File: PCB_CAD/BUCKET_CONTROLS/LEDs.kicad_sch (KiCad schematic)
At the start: 104 parts, among them J1 Pow, J10 Data, J101 Pow, J102 Data, J103 Pow, J104 Data, J105 Pow, J106 Data, J107 Pow, J108 Data, J109 Pow, J11 Pow, J110 Data, J111 Pow, J112 Data, J113 Pow, J114 Data, J115 Pow, J116 Data, J117 Pow, J118 Data, J119 Pow, J12 Data, J120 Data, J13 Pow, J14 Pow, J15 Pow, J16 Data, J17 Data, J18 Data, J19 Pow, J2 Data, J20 Data, J201 Pow, J202 Data, J203 Pow, J204 Data, J205 Pow, J206 Data, J207 Pow, J208 Data, J209 Pow, J210 Data, J211 Pow, J212 Data, J213 Pow, J214 Data, J215 Pow, J216 Data, J217 Pow, J218 Data, J219 Pow, J220 Data, J3 Pow, J301 Pow, J302 Data, J303 Pow, J304 Data, J305 Pow, J306 Data, J307 Pow, J308 Data, J309 Pow, J310 Data, J311 Pow, J312 Data, J313 Pow, J314 Data, J315 Pow, J316 Data, J317 Pow, J318 Data, J319 Pow, J320 Data, J4 Data, J5 Pow, J6 Data, J7 Pow, J8 Pow, J9 Data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

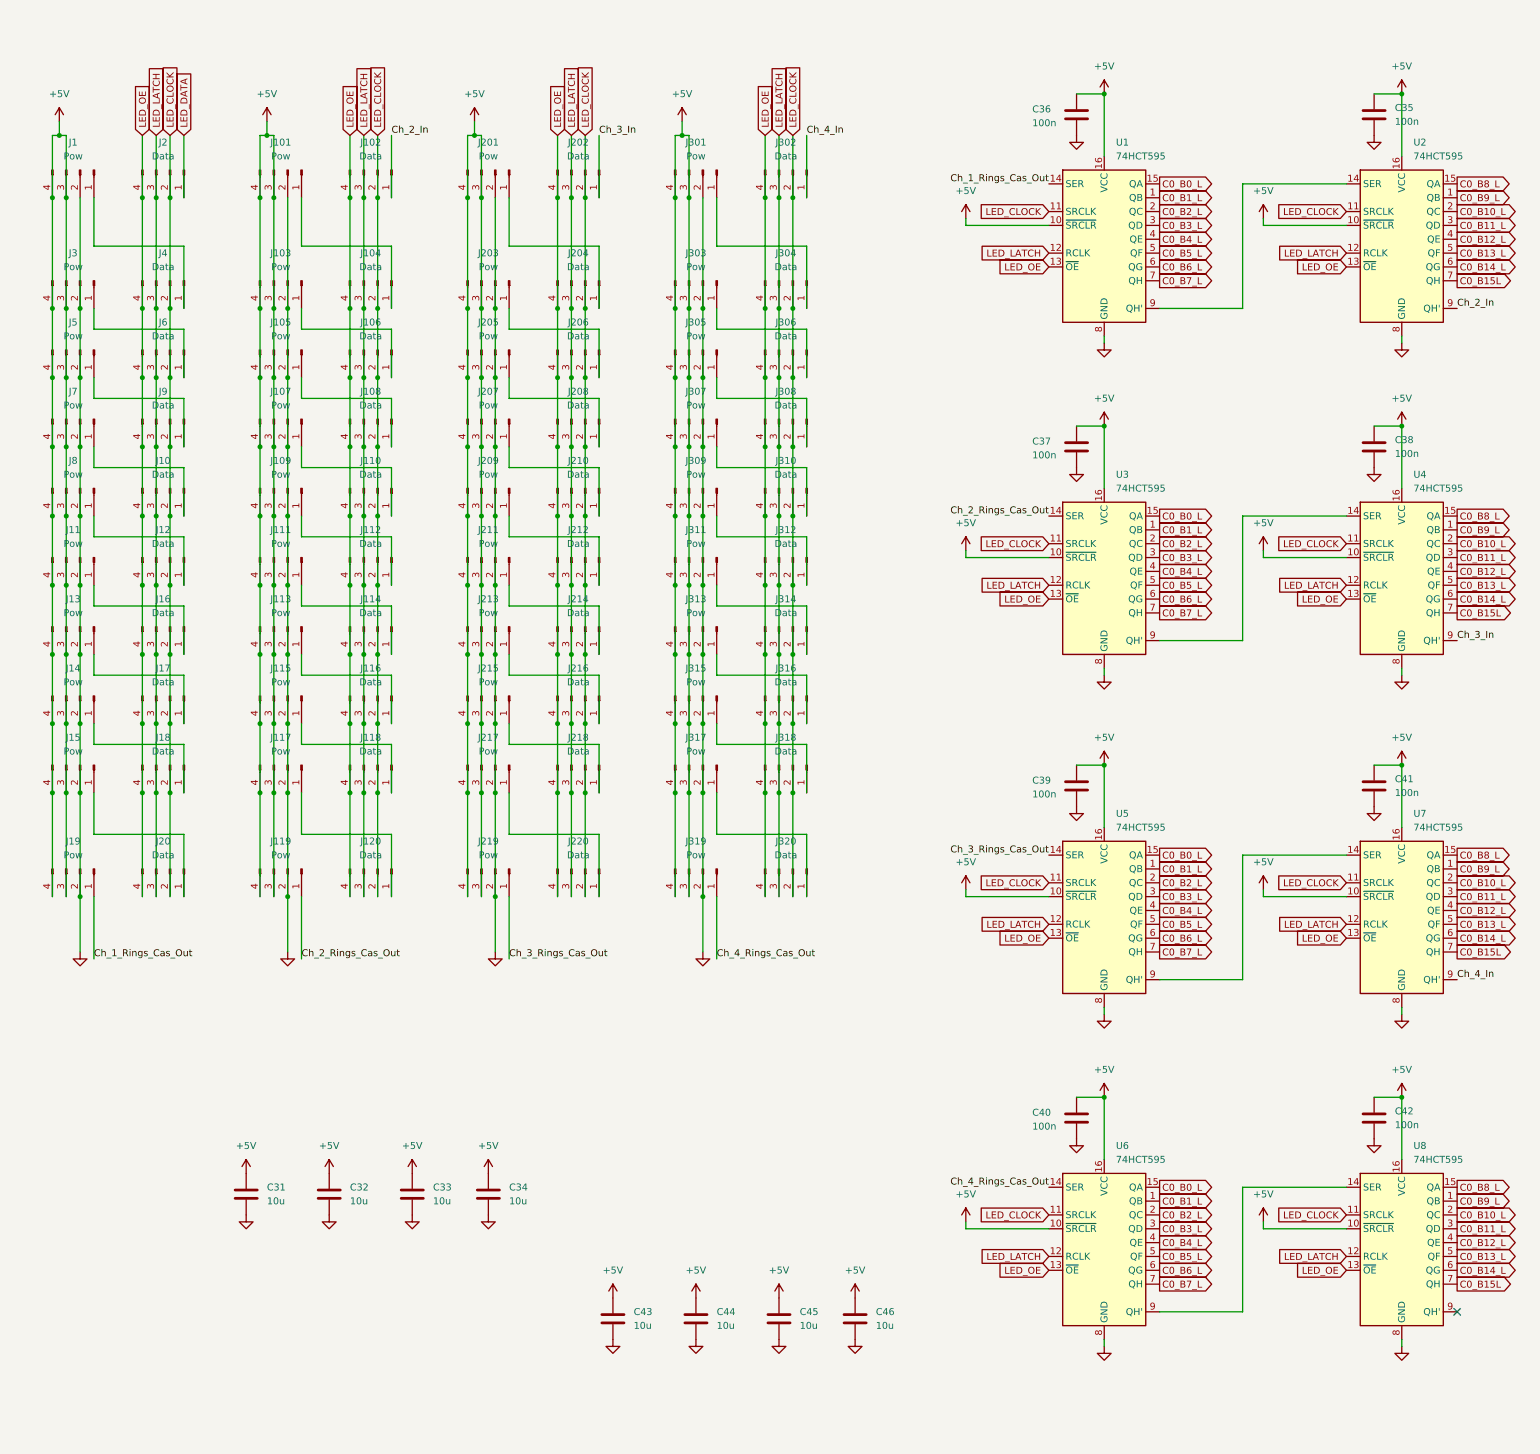
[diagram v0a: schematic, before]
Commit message: saving progress on controls pcb
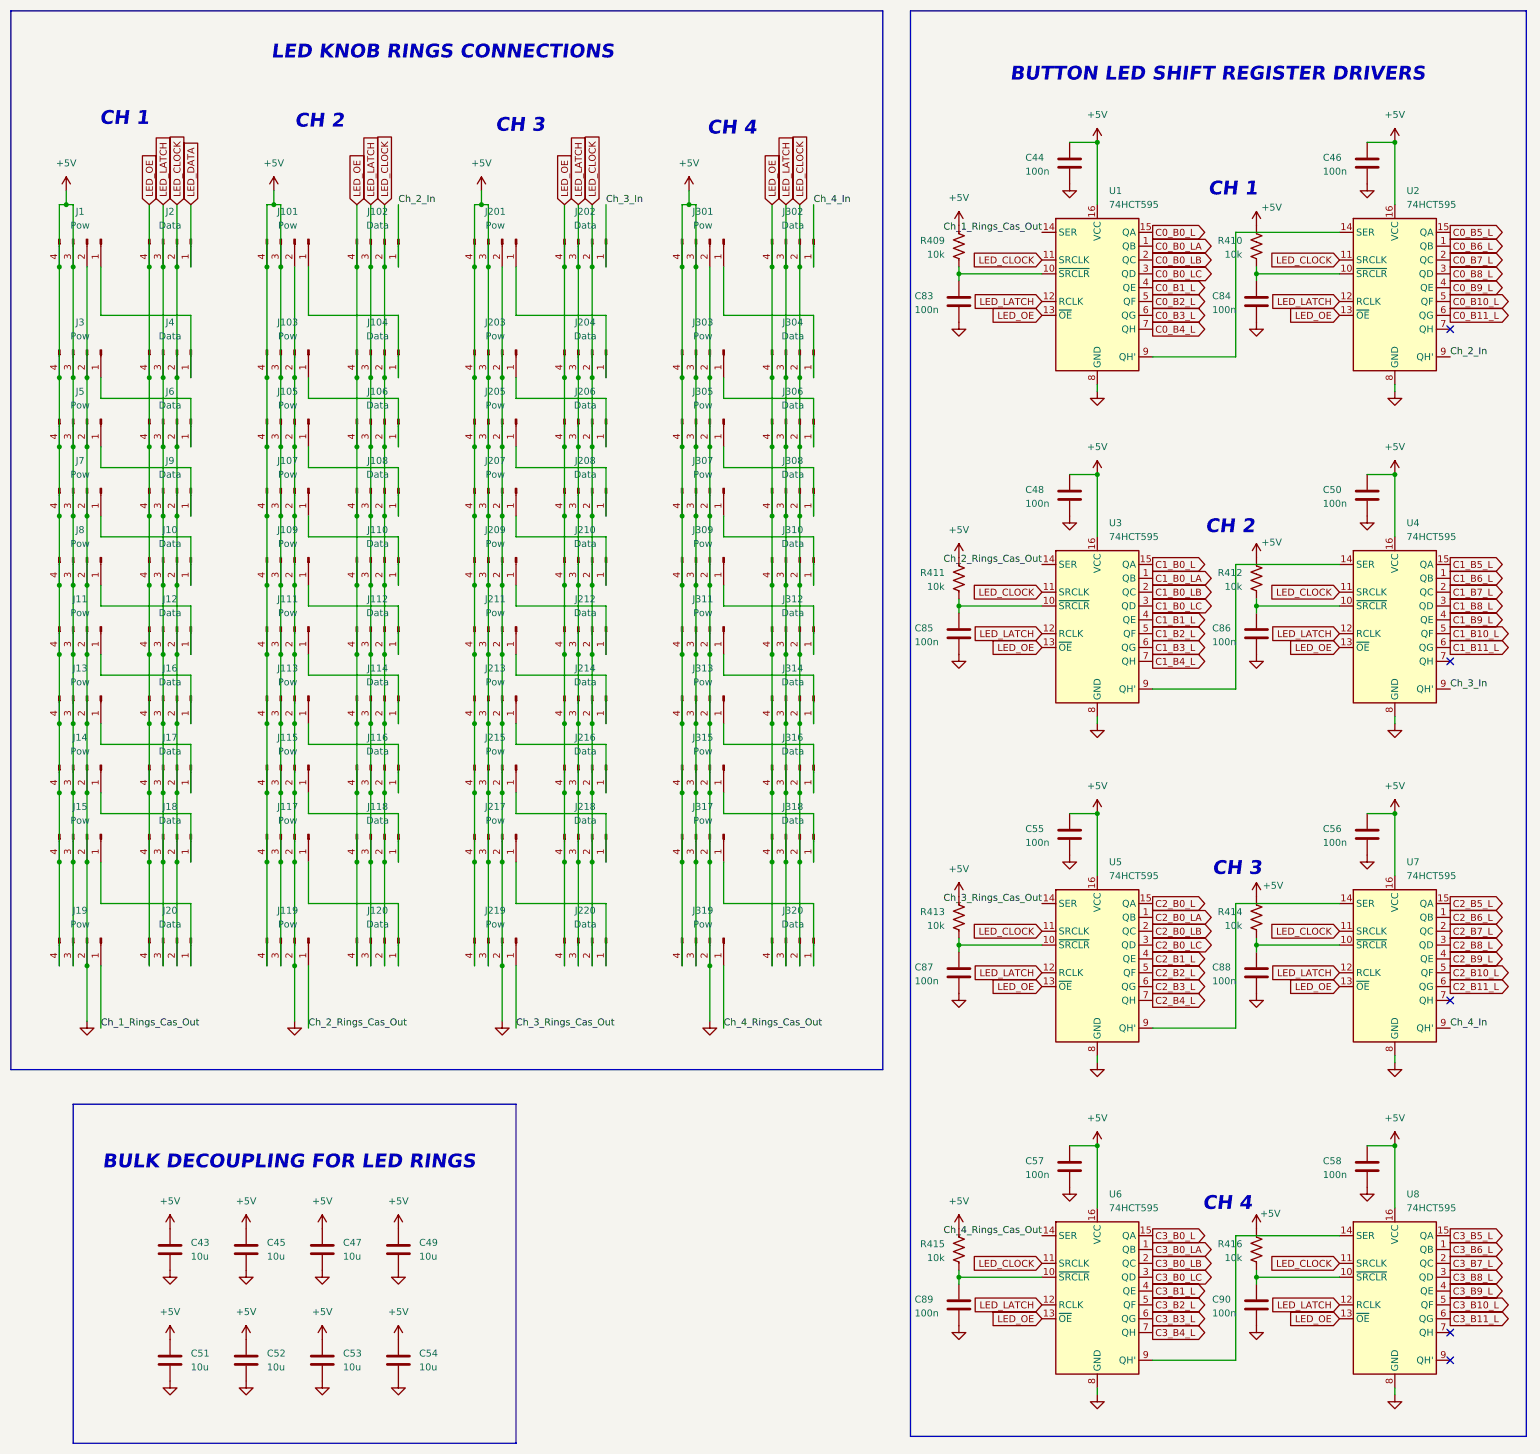
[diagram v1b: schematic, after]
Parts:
- removed C31, C32, C33, C34: 10u, Capacitor_SMD:C_0402_1005Metric, symbol Device:C
- removed C35, C36, C37, C38, C39, C40, C41, C42: 100n, Capacitor_SMD:C_0402_1005Metric, symbol Device:C
- added C47, C49, C51, C52, C53, C54: 10u, Capacitor_SMD:C_0603_1608Metric, symbol Device:C
- added C48, C50, C55, C56, C57, C58, C83, C84, C85, C86, C87, C88, C89, C90: 100n, Capacitor_SMD:C_0402_1005Metric, symbol Device:C
- added R409, R410, R411, R412, R413, R414, R415, R416: 10k, Resistor_SMD:R_0603_1608Metric, symbol Device:R_US
- C43, C45: footprint Capacitor_SMD:C_0402_1005Metric -> Capacitor_SMD:C_0603_1608Metric; LCSC C386033 -> C19702
- C44, C46: value 10u -> 100n; LCSC C386033 -> C1525
- J1, J10, J101, J102, J103, J104, J105, J106, J107, J108, J109, J11, J110, J111, J112, J113, J114, J115, J116, J117, J118, J119, J12, J120, J13, J14, J15, J16, J17, J18, J19, J2, J20, J201, J202, J203, J204, J205, J206, J207, J208, J209, J210, J211, J212, J213, J214, J215, J216, J217, J218, J219, J220, J3, J301, J302, J303, J304, J305, J306, J307, J308, J309, J310, J311, J312, J313, J314, J315, J316, J317, J318, J319, J320, J4, J5, J6, J7, J8, J9: LCSC (none) -> dnp
- U1, U2, U3, U4, U5, U6, U7, U8: footprint (none) -> Package_SO:SOIC-16_3.9x9.9mm_P1.27mm; LCSC (none) -> C282339
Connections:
- net +5V: now also C47.1, C48.1, C49.1, C50.1, C51.1, C52.1, C53.1, C54.1, C55.1, C56.1, C57.1, C58.1, R409.1, R410.1, R411.1, R412.1, R413.1, R414.1, R415.1, R416.1; no longer U1.10 (~{SRCLR}), U2.10 (~{SRCLR}), U3.10 (~{SRCLR}), U4.10 (~{SRCLR}), U5.10 (~{SRCLR}), U6.10 (~{SRCLR}), U7.10 (~{SRCLR}), U8.10 (~{SRCLR})
- net C0_B0_L: no longer U3.15 (QA), U5.15 (QA), U6.15 (QA)
- net C0_B10_L: now also U2.5 (QF); no longer U2.2 (QC), U4.2 (QC), U7.2 (QC), U8.2 (QC)
- net C0_B11_L: now also U2.6 (QG); no longer U2.3 (QD), U4.3 (QD), U7.3 (QD), U8.3 (QD)
- net C0_B1_L: now also U1.4 (QE); no longer U1.1 (QB), U3.1 (QB), U5.1 (QB), U6.1 (QB)
- net C0_B2_L: now also U1.5 (QF); no longer U1.2 (QC), U3.2 (QC), U5.2 (QC), U6.2 (QC)
- net C0_B3_L: now also U1.6 (QG); no longer U1.3 (QD), U3.3 (QD), U5.3 (QD), U6.3 (QD)
- net C0_B4_L: now also U1.7 (QH); no longer U1.4 (QE), U3.4 (QE), U5.4 (QE), U6.4 (QE)
- net C0_B5_L: now also U2.15 (QA); no longer U1.5 (QF), U3.5 (QF), U5.5 (QF), U6.5 (QF)
- net C0_B6_L: now also U2.1 (QB); no longer U1.6 (QG), U3.6 (QG), U5.6 (QG), U6.6 (QG)
- net C0_B7_L: now also U2.2 (QC); no longer U1.7 (QH), U3.7 (QH), U5.7 (QH), U6.7 (QH)
- net C0_B8_L: now also U2.3 (QD); no longer U2.15 (QA), U4.15 (QA), U7.15 (QA), U8.15 (QA)
- net C0_B9_L: now also U2.4 (QE); no longer U2.1 (QB), U4.1 (QB), U7.1 (QB), U8.1 (QB)
- net GND: now also C47.2, C48.2, C49.2, C50.2, C51.2, C52.2, C53.2, C54.2, C55.2, C56.2, C57.2, C58.2, C83.2, C84.2, C85.2, C86.2, C87.2, C88.2, C89.2, C90.2
- removed net C0_B12_L: U2.4 (QE), U4.4 (QE), U7.4 (QE), U8.4 (QE)
- removed net C0_B13_L: U2.5 (QF), U4.5 (QF), U7.5 (QF), U8.5 (QF)
- removed net C0_B14_L: U2.6 (QG), U4.6 (QG), U7.6 (QG), U8.6 (QG)
- removed net C0_B15L: U2.7 (QH), U4.7 (QH), U7.7 (QH), U8.7 (QH)
- new net: C90.1, R416.2, U8.10 (~{SRCLR})
- new net: C88.1, R414.2, U7.10 (~{SRCLR})
- new net: C89.1, R415.2, U6.10 (~{SRCLR})
- new net: C84.1, R410.2, U2.10 (~{SRCLR})
- new net: C85.1, R411.2, U3.10 (~{SRCLR})
- new net: C86.1, R412.2, U4.10 (~{SRCLR})
- new net: C87.1, R413.2, U5.10 (~{SRCLR})
- new net: C83.1, R409.2, U1.10 (~{SRCLR})
- new net C0_B0_LA: U1.1 (QB)
- new net C0_B0_LB: U1.2 (QC)
- new net C0_B0_LC: U1.3 (QD)
- new net C1_B0_L: U3.15 (QA)
- new net C1_B0_LA: U3.1 (QB)
- new net C1_B0_LB: U3.2 (QC)
- new net C1_B0_LC: U3.3 (QD)
- new net C1_B10_L: U4.5 (QF)
- new net C1_B11_L: U4.6 (QG)
- new net C1_B1_L: U3.4 (QE)
- new net C1_B2_L: U3.5 (QF)
- new net C1_B3_L: U3.6 (QG)
- new net C1_B4_L: U3.7 (QH)
- new net C1_B5_L: U4.15 (QA)
- new net C1_B6_L: U4.1 (QB)
- new net C1_B7_L: U4.2 (QC)
- new net C1_B8_L: U4.3 (QD)
- new net C1_B9_L: U4.4 (QE)
- new net C2_B0_L: U5.15 (QA)
- new net C2_B0_LA: U5.1 (QB)
- new net C2_B0_LB: U5.2 (QC)
- new net C2_B0_LC: U5.3 (QD)
- new net C2_B10_L: U7.5 (QF)
- new net C2_B11_L: U7.6 (QG)
- new net C2_B1_L: U5.4 (QE)
- new net C2_B2_L: U5.5 (QF)
- new net C2_B3_L: U5.6 (QG)
- new net C2_B4_L: U5.7 (QH)
- new net C2_B5_L: U7.15 (QA)
- new net C2_B6_L: U7.1 (QB)
- new net C2_B7_L: U7.2 (QC)
- new net C2_B8_L: U7.3 (QD)
- new net C2_B9_L: U7.4 (QE)
- new net C3_B0_L: U6.15 (QA)
- new net C3_B0_LA: U6.1 (QB)
- new net C3_B0_LB: U6.2 (QC)
- new net C3_B0_LC: U6.3 (QD)
- new net C3_B10_L: U8.5 (QF)
- new net C3_B11_L: U8.6 (QG)
- new net C3_B1_L: U6.4 (QE)
- new net C3_B2_L: U6.5 (QF)
- new net C3_B3_L: U6.6 (QG)
- new net C3_B4_L: U6.7 (QH)
- new net C3_B5_L: U8.15 (QA)
- new net C3_B6_L: U8.1 (QB)
- new net C3_B7_L: U8.2 (QC)
- new net C3_B8_L: U8.3 (QD)
- new net C3_B9_L: U8.4 (QE)
- no-connect marks 1 -> 5
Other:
- note added: "BULK DECOUPLING FOR LED RINGS"
- note added: "BUTTON LED SHIFT REGISTER DRIVERS"
- note added: "CH 1"
- note added: "CH 2"
- note added: "CH 3"
- note added: "CH 4"
- note added: "LED KNOB RINGS CONNECTIONS"
- moved on the sheet: J1, J10, J101, J102, J103, J104, J105, J106, J107, J108, J109, J11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
